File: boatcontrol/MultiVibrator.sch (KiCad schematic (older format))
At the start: 4 parts, among them IC401 CD74HCT221E

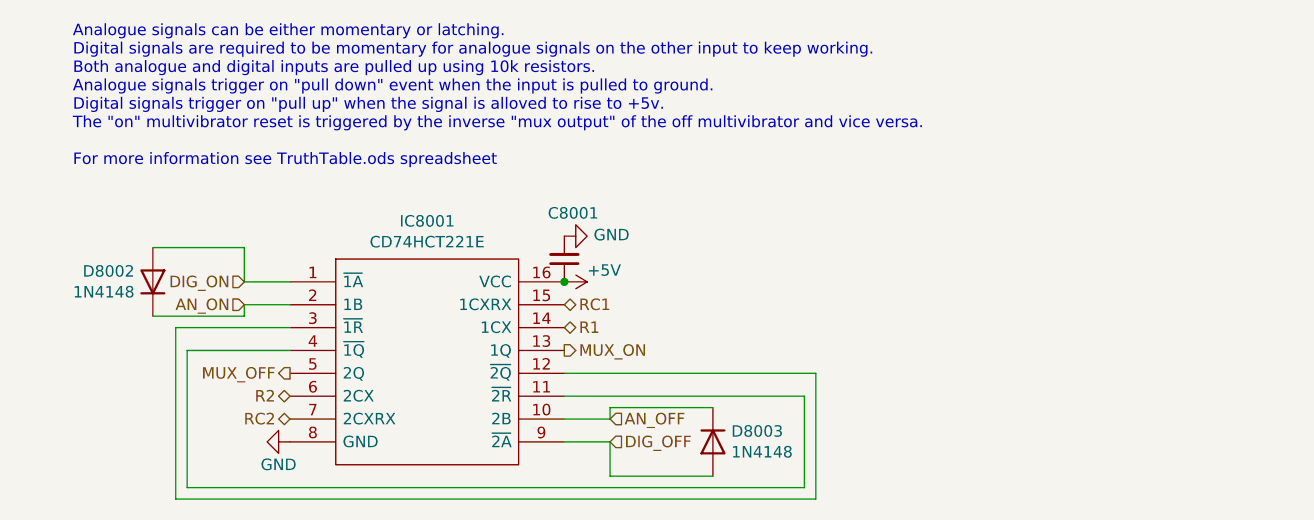
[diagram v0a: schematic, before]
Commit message: More cleanup
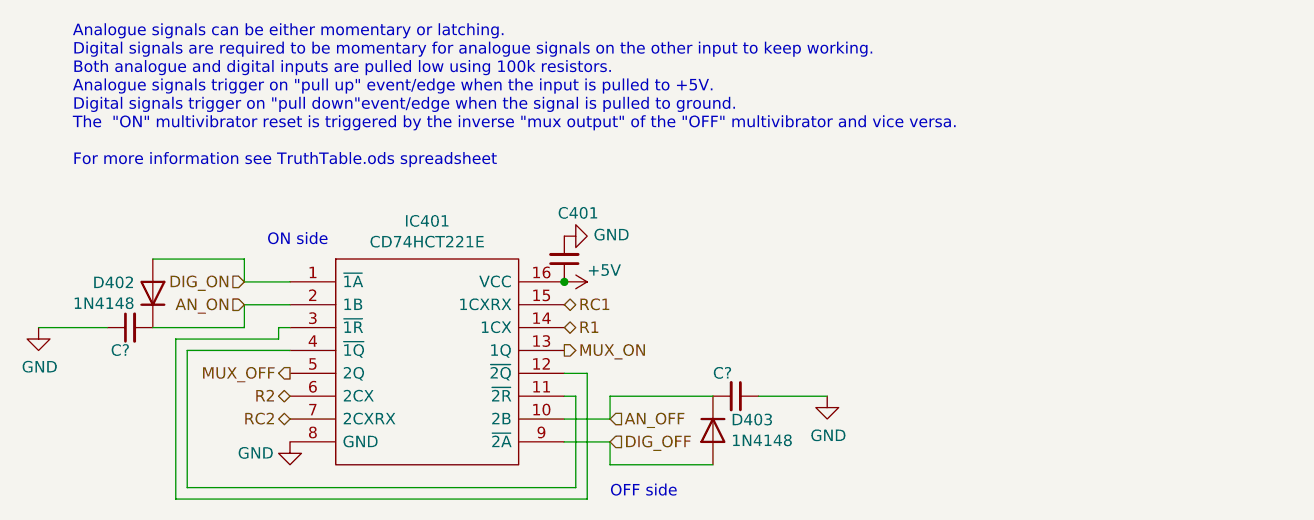
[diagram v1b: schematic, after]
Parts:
- added C? (x2): 1µF, Capacitor_THT:C_Disc_D7.5mm_W5.0mm_P5.00mm, symbol Device:C_Small
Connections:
- net AN_OFF: now also C?.2
- net AN_ON: now also C?.2
- net GND: now also C?.1, C?.1
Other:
- note added: "Analogue signals can be either momentary or latching.\nDigital signals are required to be momentary for analogue signals on the other input to keep working.\nBoth analogue and digital inputs are pulled low using 100k resistors.\nAnalogue signals trigger on "pull up" event/edge when the input is pulled to +5V.\nDigital signals trigger on "pull down"event/edge when the signal is pulled to ground.\n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"
- note added: "OFF side"
- note added: "ON side"
- note removed: "Analogue signals can be either momentary or latching.\nDigital signals are required to be momentary for analogue signals on the other input to keep working.\nBoth analogue and digital inputs are pulled up using 10k resistors.\nAnalogue signals trigger on "pull down" event when the input is pulled to ground.\nDigital signals trigger on "pull up" when the signal is alloved to rise to +5v.\nThe "on"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"
- moved on the sheet: D402, D403
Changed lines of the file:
@@
 $Descr A4 11693 8268
 encoding utf-8
-Sheet 68 97
+Sheet 10 97
 Title "Boat Control Hat"
 Date ""
@@
 $EndDescr
 Text Notes 3900 3450 0    50   ~ 0
-Analogue signals can be either momentary or latching.\nDigital signals are required to be momentary for analogue signals on the other input to keep working.\nBoth analogue and digital inputs are pulled up using 10k resistors.\nAnalogue signals trigger on "pull down" event when the input is pulled to ground.\nDigital signals trigger on "pull up" when the signal is alloved to rise to +5v.\nThe "on" multivibrator reset is triggered by the inverse "mux output" of the off multivibrator and vice versa.\n\nFor more information see TruthTable.ods spreadsheet
-Wire Wire Line
-	4400 4250 4400 4850
-Wire Wire Line
-	4850 4250 4400 4250
+Analogue signals can be either momentary or latching.\nDigital signals are required to be momentary for analogue signals on the other input to keep working.\nBoth analogue and digital inputs are pulled low using 100k resistors.\nAnalogue signals trigger on "pull up" event/edge when the input is pulled to +5V.\nDigital signals trigger on "pull down"event/edge when the signal is pulled to ground.\nThe  "ON" multivibrator reset is triggered by the inverse "mux output" of the "OFF" multivibrator and vice versa.\n\nFor more information see TruthTable.ods spreadsheet
 Wire Wire Line
 	4650 4050 4850 4050
@@
 AR Path="/D1BB8DB4/5F75E923/604747F3/5FD2B9DE" Ref="IC7301"  Part="1"
 AR Path="/D1BB8DB4/5F75E923/604747FF/5FD2B9DE" Ref="IC7401"  Part="1"
-F 0 "IC8001" H 5450 4215 50  0000 C CNN
+F 0 "IC401" H 5450 4215 50  0000 C CNN
 F 1 "CD74HCT221E" H 5450 4124 50  0000 C CNN
 F 2 "DIP794W53P254L1930H508Q16N" H 5900 4050 50  0001 L CNN
@@
 AR Path="/D1BB8DB4/5F75E923/604747F3/5FDA22CD" Ref="#PWR07302"  Part="1"
 AR Path="/D1BB8DB4/5F75E923/604747FF/5FDA22CD" Ref="#PWR07402"  Part="1"
-F 0 "#PWR08002" H 4850 4400 50  0001 C CNN
-F 1 "GND" V 4950 4600 50  0000 C CNN
+F 0 "#PWR0402" H 4850 4400 50  0001 C CNN
+F 1 "GND" H 4700 4600 50  0000 C CNN
 F 2 "" H 4850 4650 50  0001 C CNN
 F 3 "" H 4850 4650 50  0001 C CNN
 	1    4850 4650
-	0    1    1    0
+	1    0    0    -1
 $EndComp
 $Comp
@@
 AR Path="/D1BB8DB4/5F75E923/604747F3/5FD9FC74" Ref="#PWR07301"  Part="1"
 AR Path="/D1BB8DB4/5F75E923/604747FF/5FD9FC74" Ref="#PWR07401"  Part="1"
-F 0 "#PWR08001" H 6050 3800 50  0001 C CNN
+F 0 "#PWR0401" H 6050 3800 50  0001 C CNN
 F 1 "+5V" V 6000 4050 50  0000 L CNN
 F 2 "" H 6050 3950 50  0001 C CNN
@@
 Text HLabel 6250 4650 2    50   Input ~ 0
 DIG_OFF
-Wire Wire Line
-	4350 4900 4350 4150
-Wire Wire Line
-	4350 4150 4850 4150
 Connection ~ 6050 3950
 $Comp
@@
 AR Path="/D1BB8DB4/5F317CB5/60365B0F/61CAF5C8" Ref="#PWR0183"  Part="1"
 AR Path="/D1BB8DB4/5F317CB5/60365B35/61CAF5C8" Ref="#PWR0185"  Part="1"
-F 0 "#PWR0183" H 6050 3500 50  0001 C CNN
+F 0 "#PWR0155" H 6050 3500 50  0001 C CNN
 F 1 "GND" V 6055 3622 50  0000 R CNN
 F 2 "" H 6050 3750 50  0001 C CNN
@@
 AR Path="/D1BB8DB4/5F317CB5/60365B0F/61CAE2AB" Ref="C8001"  Part="1"
 AR Path="/D1BB8DB4/5F317CB5/60365B35/61CAE2AB" Ref="C8201"  Part="1"
-F 0 "C8001" H 5900 3650 50  0000 L CNN
+F 0 "C401" H 5900 3650 50  0000 L CNN
 F 1 "0.1μF" H 6141 3805 50  0001 L CNN
 F 2 "Capacitor_THT:C_Disc_D7.5mm_W5.0mm_P5.00mm" H 6050 3850 50  0001 C CNN
@@
 $EndComp
 Wire Wire Line
-	4650 4050 4650 4100
-Wire Wire Line
-	4650 3950 4650 3800
+	4650 3950 4650 3850
 $Comp
 L Diode:1N4148 D703
 U 1 1 6050CE68
-P 6700 4650
+P 6700 4600
 AR Path="/D16552B4/5FA17F38/61B95A95/6050CE68" Ref="D703"  Part="1"
 AR Path="/D16552B4/5FA17F38/61B8E927/6050CE68" Ref="D603"  Part="1"
@@
 AR Path="/D1BB8DB4/5F317CB5/60365B35/6050CE68" Ref="D8202"  Part="1"
 AR Path="/D1BB8DB4/5F317CB5/60365B41/6050CE68" Ref="D8302"  Part="1"
-F 0 "D8003" V 6654 4570 50  0000 R CNN
-F 1 "1N4148" V 6745 4570 50  0000 R CNN
-F 2 "Diode_THT:D_DO-35_SOD27_P7.62mm_Horizontal" H 6700 4475 50  0001 C CNN
-F 3 "https://assets.nexperia.com/documents/data-sheet/1N4148_1N4448.pdf" H 6700 4650 50  0001 C CNN
-	1    6700 4650
+F 0 "D403" V 6654 4520 50  0000 R CNN
+F 1 "1N4148" V 6745 4520 50  0000 R CNN
+F 2 "Diode_THT:D_DO-35_SOD27_P7.62mm_Horizontal" H 6700 4425 50  0001 C CNN
+F 3 "https://assets.nexperia.com/documents/data-sheet/1N4148_1N4448.pdf" H 6700 4600 50  0001 C CNN
+	1    6700 4600
 	0    -1   1    0
 $EndComp
@@
 L Diode:1N4148 D702
 U 1 1 604FEDB2
-P 4250 3950
+P 4250 4000
 AR Path="/D16552B4/5FA17F38/61B95A95/604FEDB2" Ref="D702"  Part="1"
 AR Path="/D16552B4/5FA17F38/61B8E927/604FEDB2" Ref="D602"  Part="1"
@@
 AR Path="/D1BB8DB4/5F317CB5/60365B35/604FEDB2" Ref="D8201"  Part="1"
 AR Path="/D1BB8DB4/5F317CB5/60365B41/604FEDB2" Ref="D8301"  Part="1"
-F 0 "D8002" V 4296 3870 50  0000 R CNN
-F 1 "1N4148" V 4205 3870 50  0000 R CNN
-F 2 "Diode_THT:D_DO-35_SOD27_P7.62mm_Horizontal" H 4250 3775 50  0001 C CNN
-F 3 "https://assets.nexperia.com/documents/data-sheet/1N4148_1N4448.pdf" H 4250 3950 50  0001 C CNN
-	1    4250 3950
+F 0 "D402" V 4296 3920 50  0000 R CNN
+F 1 "1N4148" V 4205 3920 50  0000 R CNN
+F 2 "Diode_THT:D_DO-35_SOD27_P7.62mm_Horizontal" H 4250 3825 50  0001 C CNN
+F 3 "https://assets.nexperia.com/documents/data-sheet/1N4148_1N4448.pdf" H 4250 4000 50  0001 C CNN
+	1    4250 4000
 	0    1    -1   0
 $EndComp
 Wire Wire Line
-	4650 4100 4250 4100
-Wire Wire Line
-	4650 3800 4250 3800
-Wire Wire Line
-	6250 4550 6250 4500
-Wire Wire Line
-	6250 4500 6700 4500
-Wire Wire Line
-	6700 4800 6250 4800
-Wire Wire Line
-	6250 4800 6250 4650
-Wire Wire Line
-	7100 4450 7100 4850
-Wire Wire Line
-	7100 4850 4400 4850
-Wire Wire Line
-	6050 4450 7100 4450
-Wire Wire Line
-	4350 4900 7150 4900
-Wire Wire Line
-	7150 4900 7150 4350
-Wire Wire Line
-	6050 4350 7150 4350
+	4650 4150 4250 4150
+Wire Wire Line
+	4650 3850 4250 3850
+Wire Wire Line
+	6250 4450 6700 4450
+Wire Wire Line
+	6700 4750 6250 4750
+Wire Wire Line
+	6250 4750 6250 4650
+Wire Wire Line
+	6250 4450 6250 4550
+Wire Wire Line
+	4650 4050 4650 4150
+$Comp
+L Device:C_Small C?
+U 1 1 602120C6
+P 6800 4450
+AR Path="/602120C6" Ref="C?"  Part="1"
+AR Path="/D16552B4/D2B5CDA9/602120C6" Ref="C?"  Part="1"
+AR Path="/D16552B4/D1AAA1EE/602120C6" Ref="C?"  Part="1"
+AR Path="/D16552B4/D1AAA1CA/602120C6" Ref="C?"  Part="1"
+AR Path="/D16552B4/5FA17F86/602120C6" Ref="C?"  Part="1"
+AR Path="/D16552B4/5FA17F38/602120C6" Ref="C?"  Part="1"
+AR Path="/D16552B4/5FA17F52/602120C6" Ref="C?"  Part="1"
+AR Path="/D16552B4/5FA17F6C/602120C6" Ref="C?"  Part="1"
+AR Path="/D16552B4/5FA17F38/5FC6571E/602120C6" Ref="C?"  Part="1"
+F 0 "C?" V 6900 4350 50  0000 L CNN
+F 1 "1µF" H 5950 4350 50  0001 L CNN
+F 2 "Capacitor_THT:C_Disc_D7.5mm_W5.0mm_P5.00mm" H 6800 4450 50  0001 C CNN
+F 3 "https://www.digikey.com/en/products/detail/kemet/C330C105K5R5TA7301/3726162" H 6800 4450 50  0001 C CNN
+F 4 "C330C105K5R5TA7301" V 6800 4450 50  0001 C CNN "Type"
+F 5 "1µF ±10% 50V Ceramic Capacitor X7R Radial" V 6800 4450 50  0001 C CNN "Description"
+	1    6800 4450
+	0    1    -1   0
+$EndComp
+$Comp
+L power:GND #PWR?
+U 1 1 602124D8
+P 7200 4450
+F 0 "#PWR?" H 7200 4200 50  0001 C CNN
+F 1 "GND" H 7205 4277 50  0000 C CNN
+F 2 "" H 7200 4450 50  0001 C CNN
+F 3 "" H 7200 4450 50  0001 C CNN
+	1    7200 4450
+	1    0    0    -1
+$EndComp
+Wire Wire Line
+	7200 4450 6900 4450
+$Comp
+L Device:C_Small C?
+U 1 1 6021685A
+P 4150 4150
+AR Path="/6021685A" Ref="C?"  Part="1"
+AR Path="/D16552B4/D2B5CDA9/6021685A" Ref="C?"  Part="1"
+AR Path="/D16552B4/D1AAA1EE/6021685A" Ref="C?"  Part="1"
+AR Path="/D16552B4/D1AAA1CA/6021685A" Ref="C?"  Part="1"
+AR Path="/D16552B4/5FA17F86/6021685A" Ref="C?"  Part="1"
+AR Path="/D16552B4/5FA17F38/6021685A" Ref="C?"  Part="1"
+AR Path="/D16552B4/5FA17F52/6021685A" Ref="C?"  Part="1"
+AR Path="/D16552B4/5FA17F6C/6021685A" Ref="C?"  Part="1"
+F 0 "C?" V 4250 4150 50  0000 L CNN
+F 1 "1µF" H 3300 4050 50  0001 L CNN
+F 2 "Capacitor_THT:C_Disc_D7.5mm_W5.0mm_P5.00mm" H 4150 4150 50  0001 C CNN
+F 3 "https://www.digikey.com/en/products/detail/kemet/C330C105K5R5TA7301/3726162" H 4150 4150 50  0001 C CNN
+F 4 "C330C105K5R5TA7301" V 4150 4150 50  0001 C CNN "Type"
+F 5 "1µF ±10% 50V Ceramic Capacitor X7R Radial" V 4150 4150 50  0001 C CNN "Description"
+	1    4150 4150
+	0    -1   1    0
+$EndComp
+$Comp
+L power:GND #PWR?
+U 1 1 60216860
+P 3750 4150
+F 0 "#PWR?" H 3750 3900 50  0001 C CNN
+F 1 "GND" H 3755 3977 50  0000 C CNN
+F 2 "" H 3750 4150 50  0001 C CNN
+F 3 "" H 3750 4150 50  0001 C CNN
+	1    3750 4150
+	1    0    0    -1
+$EndComp
+Wire Wire Line
+	3750 4150 4050 4150
+Wire Wire Line
+	6050 4450 6100 4450
+Wire Wire Line
+	6100 4450 6100 4850
+Wire Wire Line
+	6100 4850 4400 4850
+Wire Wire Line
+	4400 4850 4400 4250
+Wire Wire Line
+	4400 4250 4850 4250
+Wire Wire Line
+	6150 4350 6150 4900
+Wire Wire Line
+	6150 4900 4350 4900
+Wire Wire Line
+	4350 4900 4350 4200
+Wire Wire Line
+	4350 4200 4800 4200
+Wire Wire Line
+	4800 4200 4800 4150
+Wire Wire Line
+	4800 4150 4850 4150
+Wire Wire Line
+	6050 4350 6150 4350
+Text Notes 4750 3800 0    50   ~ 0
+ON side
+Text Notes 6250 4900 0    50   ~ 0
+OFF side
 $EndSCHEMATC
